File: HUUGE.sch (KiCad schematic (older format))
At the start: 3 parts

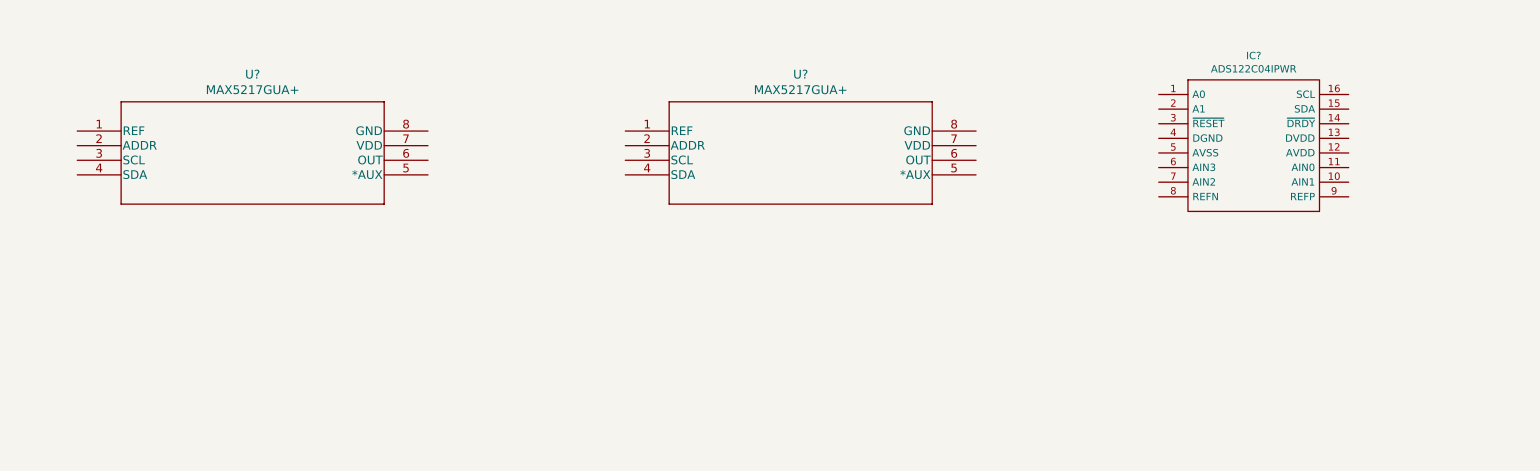
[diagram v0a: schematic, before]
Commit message: halfway
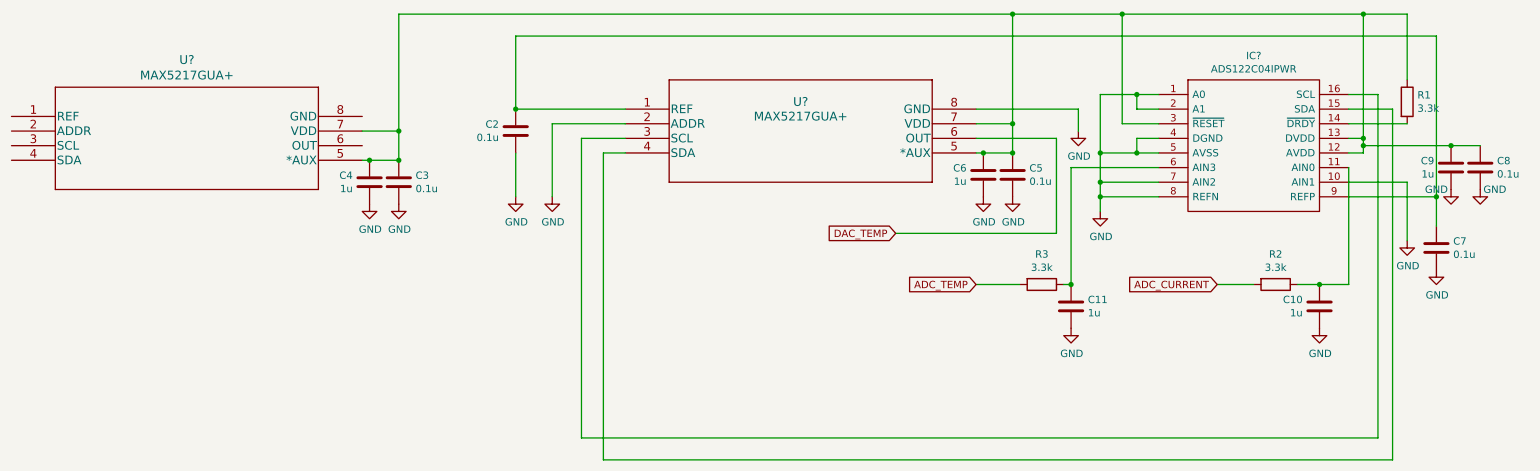
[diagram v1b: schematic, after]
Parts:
- added C10, C11, C4, C6, C9: 1u, symbol Device:C
- added C2, C3, C5, C7, C8: 0.1u, symbol Device:C
- added R1, R2, R3: 3.3k, symbol Device:R
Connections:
- net GND: now reaches IC?.1 (A0)
- net GND: now also IC?.10 (AIN1), IC?.2 (A1), IC?.4 (DGND), IC?.5 (AVSS), IC?.7 (AIN2), IC?.8 (REFN), U?.2 (ADDR), U?.8 (GND), C10.2, C11.2, C2.2, C3.2, C4.2, C5.2, C6.2, C7.2, C8.2, C9.2
- net at IC?.11 (AIN0): now also C10.1, R2.1
- net at IC?.12 (AVDD): now also IC?.13 (DVDD), IC?.3 (~RESET), U?.5 (*AUX), U?.5 (*AUX), U?.7 (VDD), U?.7 (VDD), C3.1, C4.1, C5.1, C6.1, C8.1, C9.1, R1.1
- net at IC?.14 (~DRDY): now also R1.2
- net at IC?.15 (SDA): now also U?.4 (SDA)
- net at IC?.16 (SCL): now also U?.3 (SCL)
- net at IC?.6 (AIN3): now also C11.1, R3.1
- net at IC?.9 (REFP): now also U?.1 (REF), C2.1, C7.1
- net DAC_TEMP: now reaches U?.6 (OUT)
- new net ADC_CURRENT: R2.2
- new net ADC_TEMP: R3.2
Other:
- moved on the sheet: U?
